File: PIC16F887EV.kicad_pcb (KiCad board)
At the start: 2 copper layers, 100 x 100 mm, 101 parts, among them J1 USB_C_Receptacle_USB2.0_14P, Q1 2N3904, Q2 2N3904, Q3 2N3904, Q5 2N3904, SW1 SW_Push, SW10 SW_Push, SW11 SW_Push, SW12 SW_Push, SW13 SW_Push, SW14 SW_Push, SW15 SW_Push, SW16 SW_Push, SW17 SW_Push, SW18 SW_Push, SW2 SW_Push, SW3 SW_Push, SW4 SW_Push, SW5 SW_Push, SW6 SW_Push, SW7 SW_Push, SW8 SW_Push, SW9 SW_Push, U1 PIC16F887-IP, U2 FT230XS, Y1 Crystal

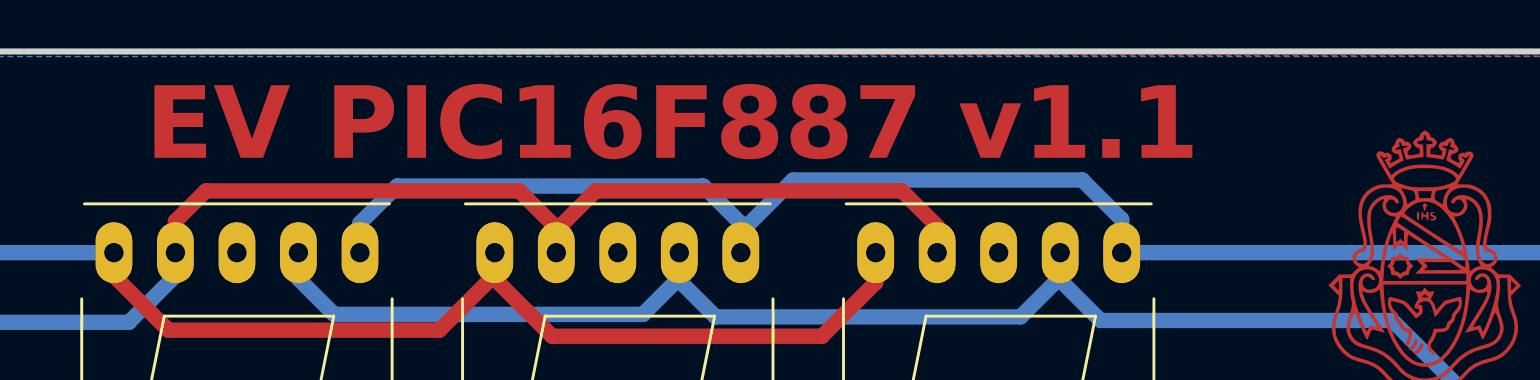
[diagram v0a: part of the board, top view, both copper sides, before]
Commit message: Cambio de nombre v2.0
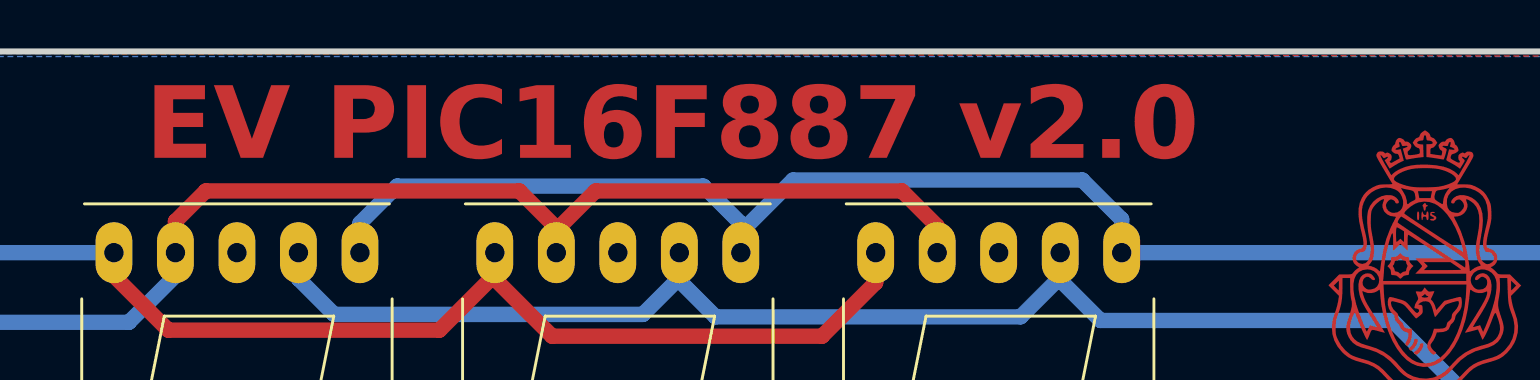
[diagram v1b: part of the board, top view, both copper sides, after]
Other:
- board text added: "EV PIC16F887 v2.0"
- board text removed: "EV PIC16F887 v1.1"
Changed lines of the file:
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@@
 		(fp_arc
 			(start -2.1747 0.3223)
-			(mid -1.600348 -4.921578)
+			(mid -1.600349 -4.921577)
 			(end 3.1903 -2.713)
 			(stroke
@@
 		(fp_arc
 			(start -2.1747 0.3223)
-			(mid -1.600348 -4.921578)
+			(mid -1.600349 -4.921577)
 			(end 3.1903 -2.713)
 			(stroke
@@
 		)
 	)
-	(gr_text "EV PIC16F887 v1.1"
+	(gr_text "EV PIC16F887 v2.0"
 		(at 43 20 0)
 		(layer "F.Cu")
@@
 		)
 	)
-	(gr_text "EV PIC16F887 v1.1"
+	(gr_text "EV PIC16F887 v2.0"
 		(at 43 20 0)
 		(layer "F.Mask")

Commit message: Revert "Cambio de nombre v2.0"
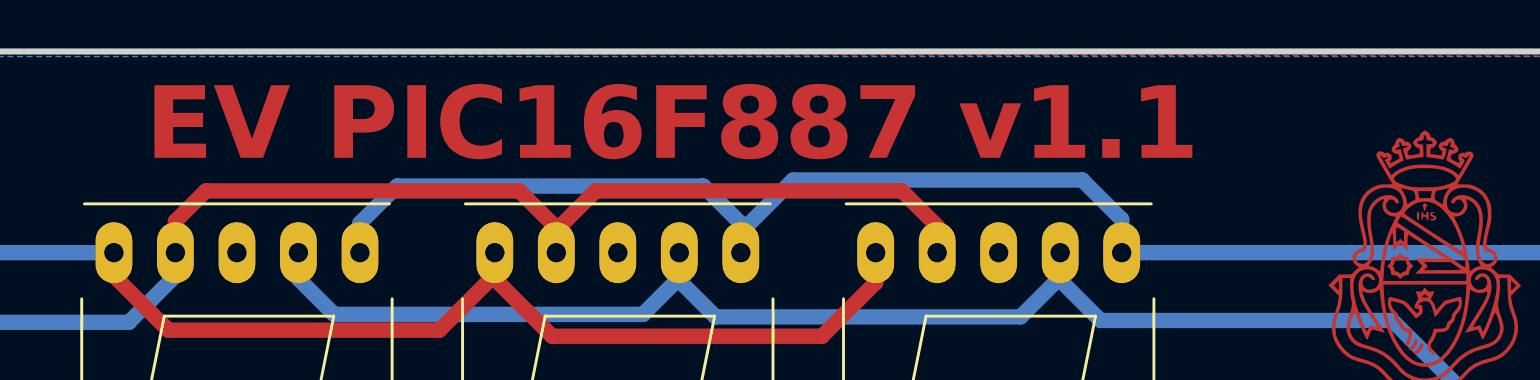
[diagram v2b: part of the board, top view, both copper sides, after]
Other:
- board text added: "EV PIC16F887 v1.1"
- board text removed: "EV PIC16F887 v2.0"
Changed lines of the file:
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@@
 		(fp_arc
 			(start -2.1747 0.3223)
-			(mid -1.600349 -4.921577)
+			(mid -1.600348 -4.921578)
 			(end 3.1903 -2.713)
 			(stroke
@@
 		(fp_arc
 			(start -2.1747 0.3223)
-			(mid -1.600349 -4.921577)
+			(mid -1.600348 -4.921578)
 			(end 3.1903 -2.713)
 			(stroke
@@
 		)
 	)
-	(gr_text "EV PIC16F887 v2.0"
+	(gr_text "EV PIC16F887 v1.1"
 		(at 43 20 0)
 		(layer "F.Cu")
@@
 		)
 	)
-	(gr_text "EV PIC16F887 v2.0"
+	(gr_text "EV PIC16F887 v1.1"
 		(at 43 20 0)
 		(layer "F.Mask")
